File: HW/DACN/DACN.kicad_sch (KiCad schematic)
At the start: 5 parts, among them J2 Conn_02x15_Counter_Clockwise, J3 PINHD_1x4_Male, J4 DC-005

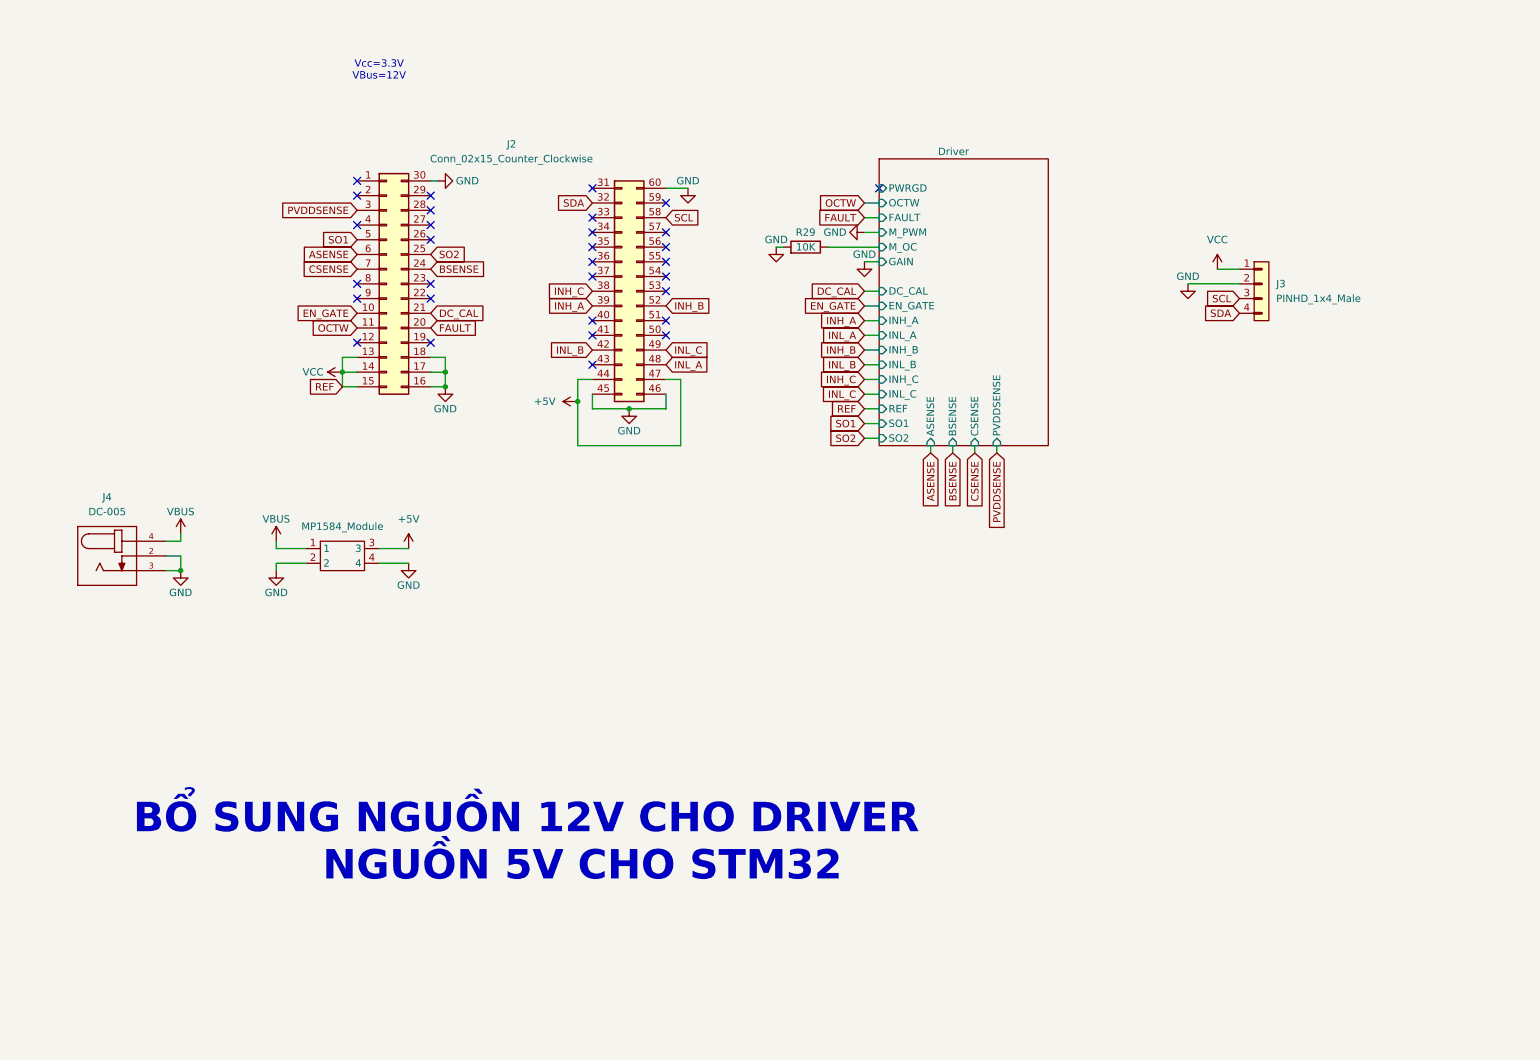
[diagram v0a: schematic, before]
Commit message: .
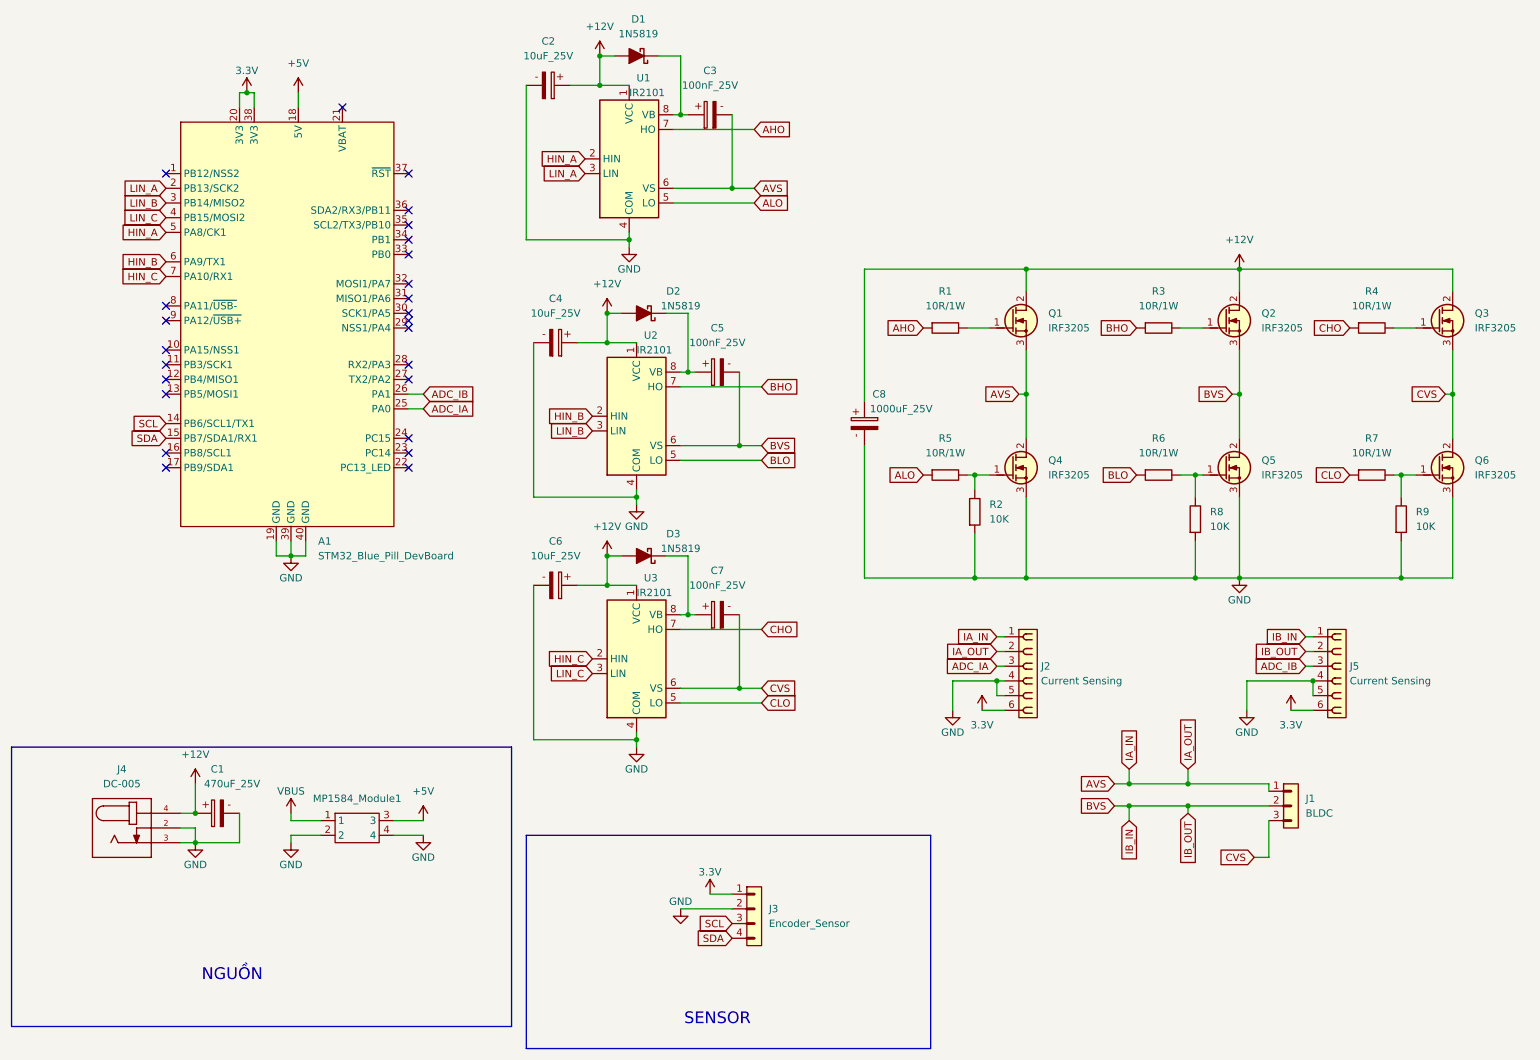
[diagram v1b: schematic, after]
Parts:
- removed J2: Conn_02x15_Counter_Clockwise, Connector_PinSocket_2.54mm:Weact_STM32F405, symbol Connector_Generic:Conn_02x15_Counter_Clockwise
- removed R29: 10K, PCM_Resistor_SMD_AKL:R_0805_2012Metric, symbol PCM_Resistor_AKL:R_0805
- added A1: STM32_Blue_Pill_DevBoard, PCM_SL_Development_Boards:STM32_Blue_Pill_DevBoard, symbol PCM_SL_Development_Board:STM32_Blue_Pill_DevBoard
- added C1: 470uF_25V, Capacitor_THT:CP_Radial_D8.0mm_P3.50mm, symbol PCM_SL_Capacitors:470uF_25V
- added C2, C4, C6: 10uF_25V, Capacitor_THT:CP_Radial_D5.0mm_P2.00mm, symbol PCM_SL_Capacitors:10uF_25V
- added C3, C5, C7: 100nF_25V, Capacitor_THT:CP_Radial_D4.0mm_P1.50mm, symbol PCM_SL_Capacitors:1uF_50V
- added C8: 1000uF_25V, Capacitor_THT:CP_Radial_D5.0mm_P2.00mm, symbol PCM_SL_Capacitors:10uF_25V
- added D1, D2, D3: 1N5819, PCM_Diode_THT_AKL:D_DO-41_SOD81_P7.62mm_Horizontal, symbol PCM_Diode_Schottky_AKL:1N5819
- added J1: BLDC, Connector_PinHeader_2.54mm:PinHeader_1x03_P2.54mm_Vertical, symbol PCM_SL_Pin_Headers:PINHD_1x3_Male
- added J2, J5: Current Sensing, Connector_PinSocket_2.54mm:PinSocket_1x06_P2.54mm_Vertical, symbol PCM_SL_Pin_Headers:PINHD_1x6_Female
- added Q1, Q2, Q3, Q4, Q5, Q6: IRF3205, PCM_Package_TO_SOT_THT_AKL:TO-220-3_Vertical_GDS, symbol PCM_Transistor_MOSFET_AKL:IRF3205
- added R1, R3, R4, R5, R6, R7: 10R/1W, Resistor_THT:R_Axial_DIN0207_L6.3mm_D2.5mm_P10.16mm_Horizontal, symbol PCM_SL_Resistors:Resistor
- added R2, R8, R9: 10K, Resistor_THT:R_Axial_DIN0207_L6.3mm_D2.5mm_P10.16mm_Horizontal, symbol PCM_SL_Resistors:Resistor
- added U1, U2, U3: IR2101, Package_DIP:DIP-8_W10.16mm, symbol Driver_FET:IR2101
- J3: value PINHD_1x4_Male -> Encoder_Sensor
- MP1584_Module1: renamed from MP1584_Module; footprint (none) -> MP1584EN-master:SRT_MPT1584EN_Module
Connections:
- net +5V: now also A1.18 (5V)
- net GND: now also A1.19 (GND), A1.39 (GND), A1.40 (GND), C1.2, C2.2, C4.2, C6.2, C8.2, J2.4, J2.5, J5.4, J5.5, Q4.3 (S), Q5.3 (S), Q6.3 (S), R2.1, R8.1, R9.1, U1.4 (COM), U2.4 (COM), U3.4 (COM)
- net SCL: now also A1.14 (PB6/SCL1/TX1)
- net SDA: now also A1.15 (PB7/SDA1/RX1)
- net VBUS: no longer J4.4
- net VCC renamed 3.3V
- net 3.3V: now also A1.20 (3V3), A1.38 (3V3), J2.6, J5.6
- new net: C7.1, D3.1 (K), U3.8 (VB)
- new net: Q3.1 (G), R4.2
- new net: C5.1, D2.1 (K), U2.8 (VB)
- new net: C3.1, D1.1 (K), U1.8 (VB)
- new net: Q5.1 (G), R6.2, R8.2
- new net: Q6.1 (G), R7.2, R9.2
- new net: Q4.1 (G), R2.2, R5.2
- new net: Q2.1 (G), R3.2
- new net: Q1.1 (G), R1.2
- new net +12V: C1.1, C2.1, C4.1, C6.1, C8.1, D1.2 (A), D2.2 (A), D3.2 (A), J4.4, Q1.2 (D), Q2.2 (D), Q3.2 (D), U1.1 (VCC), U2.1 (VCC), U3.1 (VCC)
- new net ADC_IA: A1.25 (PA0), J2.3
- new net ADC_IB: A1.26 (PA1), J5.3
- new net AHO: R1.1, U1.7 (HO)
- new net ALO: R5.1, U1.5 (LO)
- new net AVS: C3.2, J1.1, J2.1, J2.2, Q1.3 (S), Q4.2 (D), U1.6 (VS)
- new net BHO: R3.1, U2.7 (HO)
- new net BLO: R6.1, U2.5 (LO)
- new net BVS: C5.2, J1.2, J5.1, J5.2, Q2.3 (S), Q5.2 (D), U2.6 (VS)
- new net CHO: R4.1, U3.7 (HO)
- new net CLO: R7.1, U3.5 (LO)
- new net CVS: C7.2, J1.3, Q3.3 (S), Q6.2 (D), U3.6 (VS)
- new net HIN_A: A1.5 (PA8/CK1), U1.2 (HIN)
- new net HIN_B: A1.6 (PA9/TX1), U2.2 (HIN)
- new net HIN_C: A1.7 (PA10/RX1), U3.2 (HIN)
- new net LIN_A: A1.2 (PB13/SCK2), U1.3 (LIN)
- new net LIN_B: A1.3 (PB14/MISO2), U2.3 (LIN)
- new net LIN_C: A1.4 (PB15/MOSI2), U3.3 (LIN)
- no-connect marks 31 -> 25
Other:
- removed sheet Driver
- note added: "NGUỒN"
- note added: "SENSOR"
- note removed: "BỔ SUNG NGUỒN 12V CHO DRIVER NGUỒN 5V CHO STM32"
- note removed: "Vcc=3.3V VBus=12V"
- moved on the sheet: J3, J4, MP1584_Module1
